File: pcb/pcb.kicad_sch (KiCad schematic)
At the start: 46 parts, among them J1 Power, Q1 Q_NPN_BCE, SW1 START, SW2 RESET, U1 PIC16F18346-P, U2 74HC595, U3 SCORE 1, U4 74HC595, U5 SCORE 1, U6 SSD1306

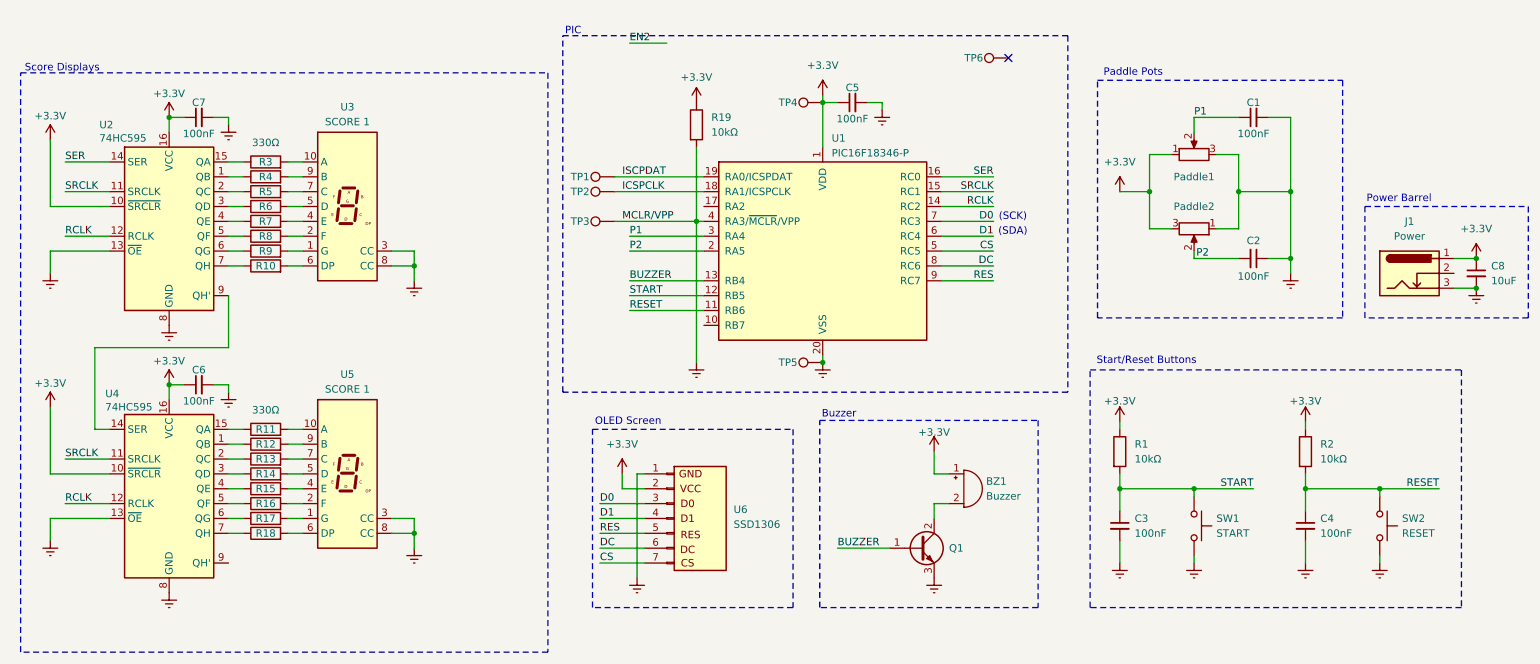
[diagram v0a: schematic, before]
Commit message: Add ball update subroutines
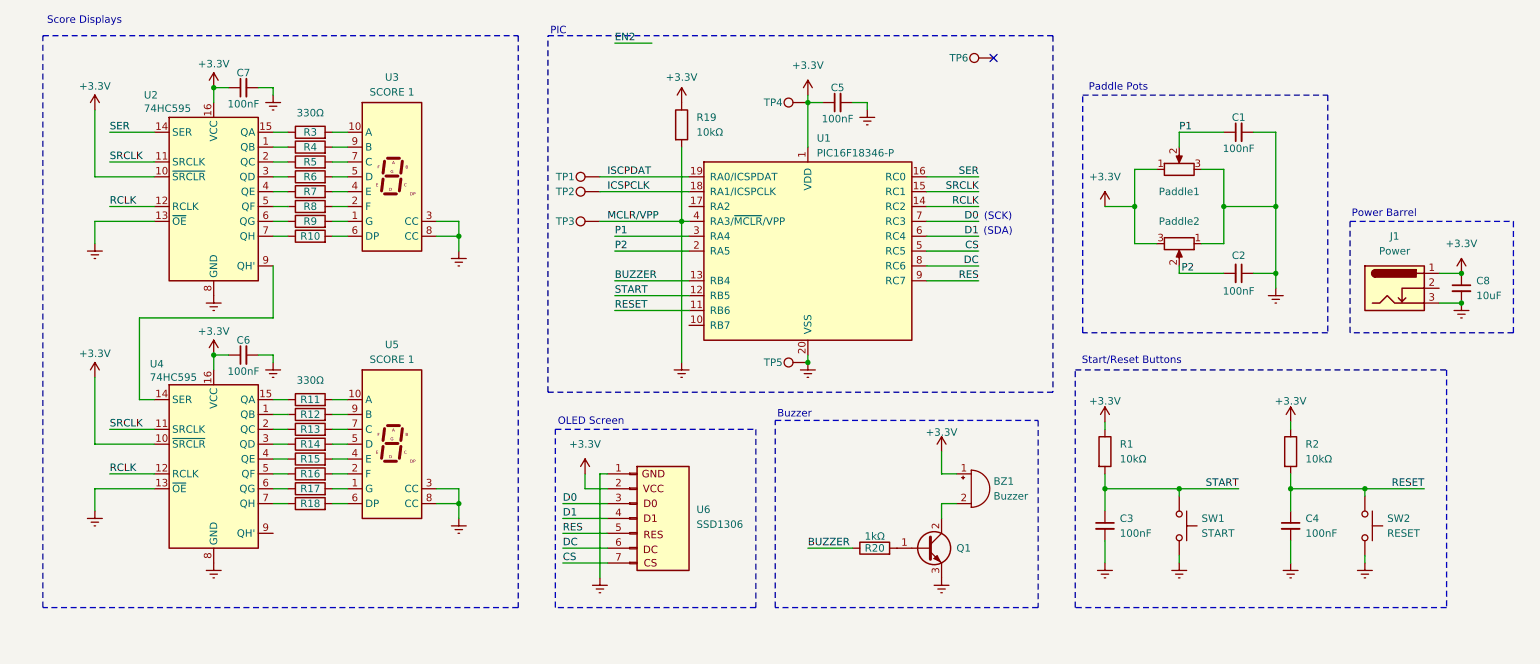
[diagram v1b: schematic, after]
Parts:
- added R20: 1kΩ, symbol Device:R
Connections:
- net BUZZER: now also R20.1; no longer Q1.1 (B)
- new net: Q1.1 (B), R20.2
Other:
- company: (none) -> tecknet-gg, jeevan hatti
- title: (none) -> asm-pong
- moved on the sheet: BZ1, C1, C2, C3, C4, C5, C6, C7, C8, J1, Paddle1, Paddle2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
